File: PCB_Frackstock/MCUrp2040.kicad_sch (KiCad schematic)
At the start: 32 parts, among them J10 SWD, J6 Conn_01x02_Male, J8 Conn_01x02_Male, U1 RP2040, U2 W25Q128JVSIQ, Y3 12MHz

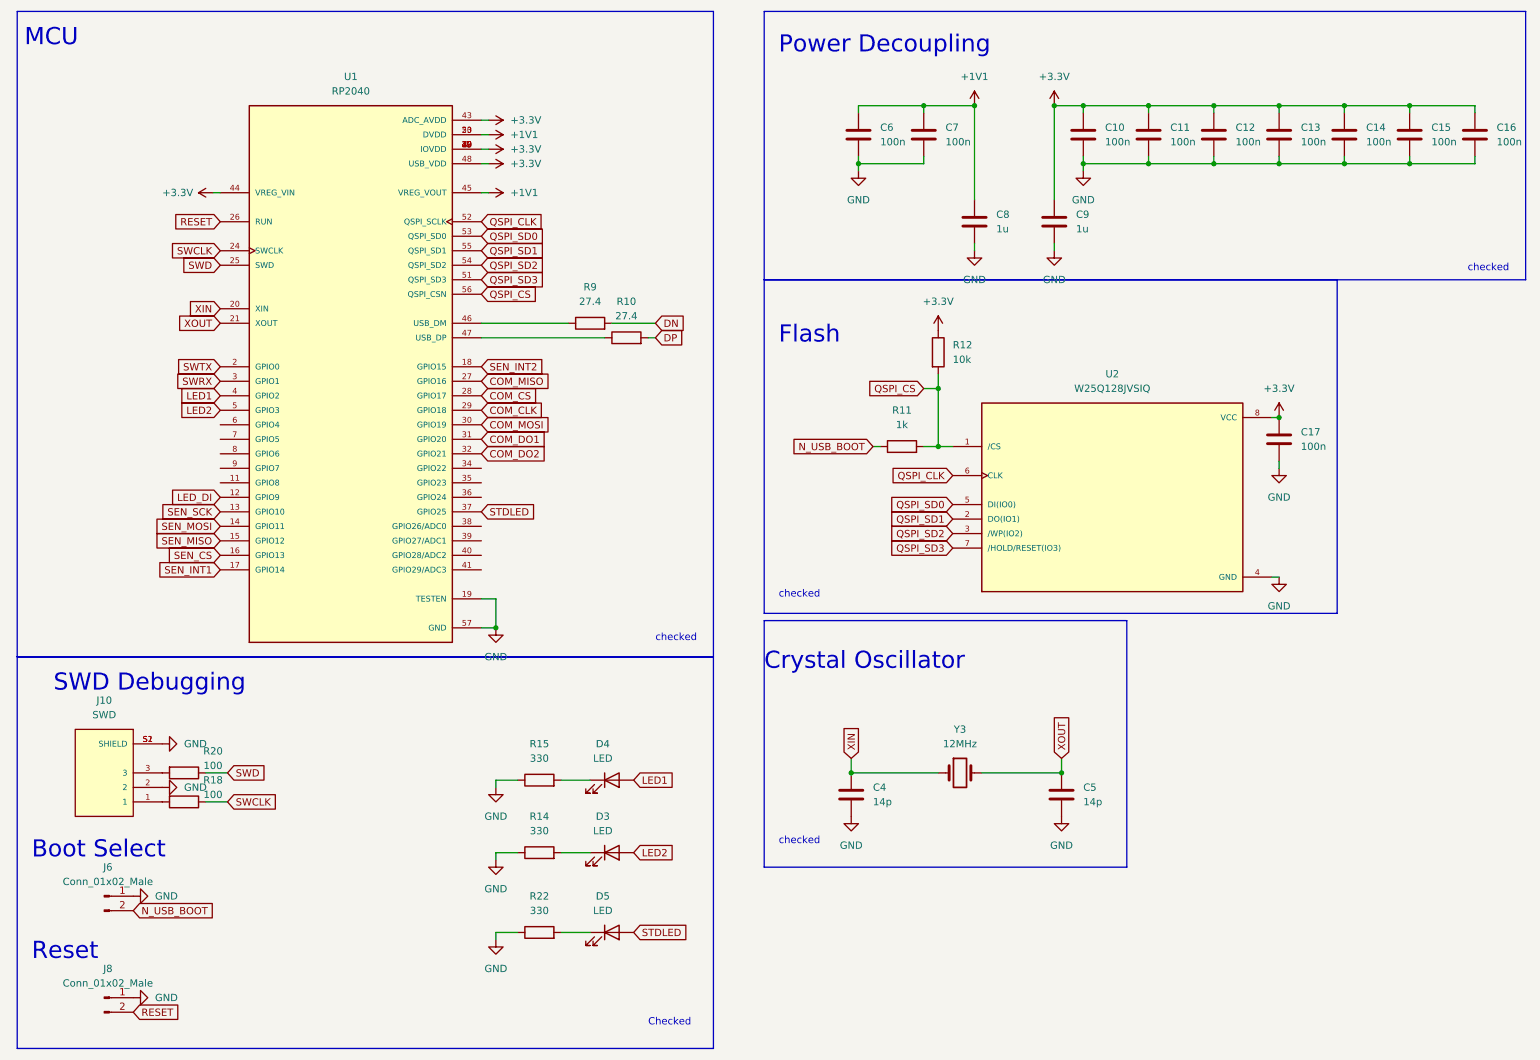
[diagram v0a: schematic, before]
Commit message: Schema_fertig
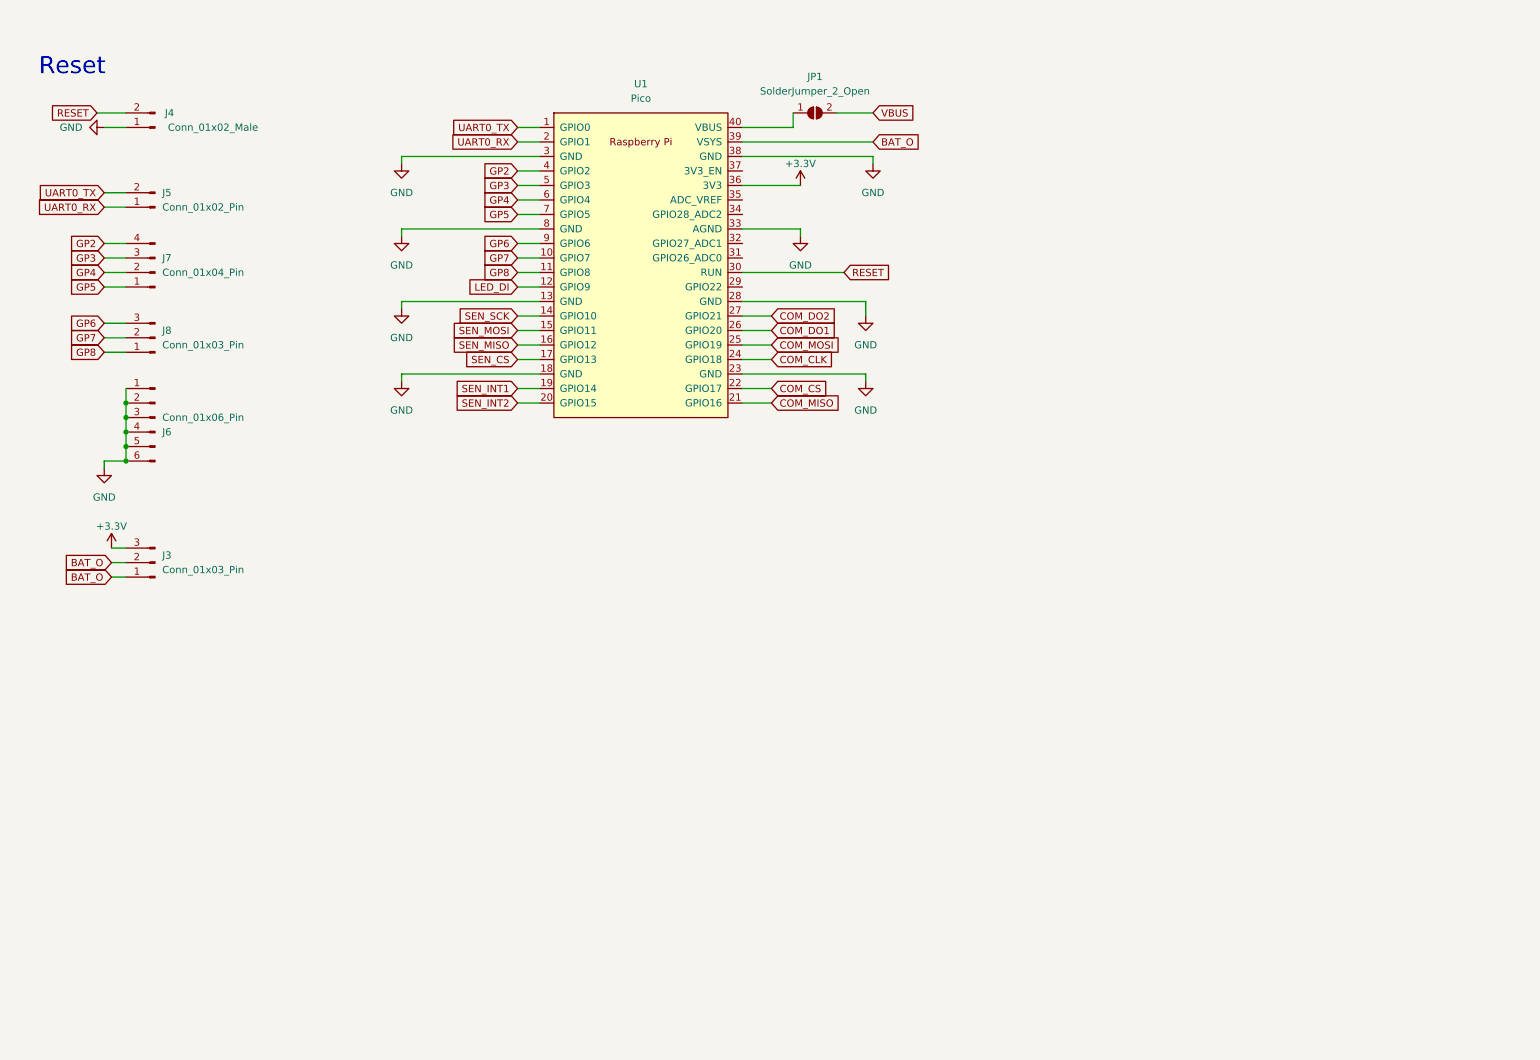
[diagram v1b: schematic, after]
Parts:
- removed C10, C11, C12, C13, C14, C15, C16, C17, C6, C7: 100n, Capacitor_SMD:C_0603_1608Metric_Pad1.08x0.95mm_HandSolder, symbol Device:C
- removed C4, C5: 14p, Capacitor_SMD:C_0603_1608Metric_Pad1.08x0.95mm_HandSolder, symbol Device:C
- removed C8, C9: 1u, Capacitor_SMD:C_0603_1608Metric_Pad1.08x0.95mm_HandSolder, symbol Device:C
- removed D3, D4, D5: LED, LED_SMD:LED_0603_1608Metric_Pad1.05x0.95mm_HandSolder, symbol Device:LED
- removed J10: SWD, SnapEDA Library:JST_SM03B-SRSS-TB(LF)(SN), symbol SM03B-SRSS-TB_LF__SN_:SM03B-SRSS-TB(LF)(SN)
- removed J6, J8: Conn_01x02_Male, Connector_PinHeader_2.54mm:PinHeader_1x02_P2.54mm_Vertical, symbol Connector:Conn_01x02_Male
- removed R10, R9: 27.4, Resistor_SMD:R_0603_1608Metric_Pad0.98x0.95mm_HandSolder, symbol Device:R
- removed R11: 1k, Resistor_SMD:R_0603_1608Metric_Pad0.98x0.95mm_HandSolder, symbol Device:R
- removed R12: 10k, Resistor_SMD:R_0603_1608Metric_Pad0.98x0.95mm_HandSolder, symbol Device:R
- removed R14, R15, R22: 330, Resistor_SMD:R_0603_1608Metric_Pad0.98x0.95mm_HandSolder, symbol Device:R
- removed R18, R20: 100, Resistor_SMD:R_0603_1608Metric_Pad0.98x0.95mm_HandSolder, symbol Device:R
- removed U1: RP2040, SnapEDA Library:QFN40P700X700X90-57N, symbol RP2040:RP2040
- removed U2: W25Q128JVSIQ, SnapEDA Library:SOIC127P790X216-8N, symbol W25Q128JVSIQ:W25Q128JVSIQ
- removed Y3: 12MHz, Crystal:Crystal_SMD_5032-2Pin_5.0x3.2mm, symbol Device:Crystal
- added J3, J8: Conn_01x03_Pin, Connector_PinHeader_2.54mm:PinHeader_1x03_P2.54mm_Vertical, symbol Connector:Conn_01x03_Pin
- added J4: Conn_01x02_Male, Connector_PinHeader_2.54mm:PinHeader_1x02_P2.54mm_Vertical, symbol Connector:Conn_01x02_Male
- added J5: Conn_01x02_Pin, Connector_PinHeader_2.54mm:PinHeader_1x02_P2.54mm_Vertical, symbol Connector:Conn_01x02_Pin
- added J6: Conn_01x06_Pin, Connector_PinHeader_2.54mm:PinHeader_1x06_P2.54mm_Vertical, symbol Connector:Conn_01x06_Pin
- added J7: Conn_01x04_Pin, Connector_PinHeader_2.54mm:PinHeader_1x04_P2.54mm_Vertical, symbol Connector:Conn_01x04_Pin
- added JP1: SolderJumper_2_Open, Jumper:SolderJumper-2_P1.3mm_Open_RoundedPad1.0x1.5mm, symbol Jumper:SolderJumper_2_Open
- added U1: Pico, Frack:RPi_Pico_SMD_ohne_Debug, symbol Frack:Pico_ohne_Debug
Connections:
- net +3.3V: now also J3.3 (Pin_3), U1.36 (3V3)
- net COM_CLK: now also U1.24 (GPIO18)
- net COM_CS: now also U1.22 (GPIO17)
- net COM_DO1: now also U1.26 (GPIO20)
- net COM_DO2: now also U1.27 (GPIO21)
- net COM_MISO: now also U1.21 (GPIO16)
- net COM_MOSI: now also U1.25 (GPIO19)
- net GND: now also J4.1 (Pin_1), J6.1 (Pin_1), J6.2 (Pin_2), J6.3 (Pin_3), J6.4 (Pin_4), J6.5 (Pin_5), J6.6 (Pin_6), U1.13 (GND), U1.18 (GND), U1.23 (GND), U1.28 (GND), U1.3 (GND), U1.33 (AGND), U1.38 (GND), U1.8 (GND)
- net LED_DI: now also U1.12 (GPIO9)
- net RESET: now also J4.2 (Pin_2), U1.30 (RUN)
- net SEN_CS: now also U1.17 (GPIO13)
- net SEN_INT1: now also U1.19 (GPIO14)
- net SEN_INT2: now also U1.20 (GPIO15)
- net SEN_MISO: now also U1.16 (GPIO12)
- net SEN_MOSI: now also U1.15 (GPIO11)
- net SEN_SCK: now also U1.14 (GPIO10)
- new net: JP1.1 (A), U1.40 (VBUS)
- new net BAT_O: J3.1 (Pin_1), J3.2 (Pin_2), U1.39 (VSYS)
- new net GP2: J7.4 (Pin_4), U1.4 (GPIO2)
- new net GP3: J7.3 (Pin_3), U1.5 (GPIO3)
- new net GP4: J7.2 (Pin_2), U1.6 (GPIO4)
- new net GP5: J7.1 (Pin_1), U1.7 (GPIO5)
- new net GP6: J8.3 (Pin_3), U1.9 (GPIO6)
- new net GP7: J8.2 (Pin_2), U1.10 (GPIO7)
- new net GP8: J8.1 (Pin_1), U1.11 (GPIO8)
- new net UART0_RX: J5.1 (Pin_1), U1.2 (GPIO1)
- new net UART0_TX: J5.2 (Pin_2), U1.1 (GPIO0)
- new net VBUS: JP1.2 (B)
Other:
- note removed: "Boot Select"
- note removed: "Checked"
- note removed: "Crystal Oscillator"
- note removed: "Flash"
- note removed: "MCU"
- note removed: "Power Decoupling"
- note removed: "SWD Debugging"
- note removed: "checked"

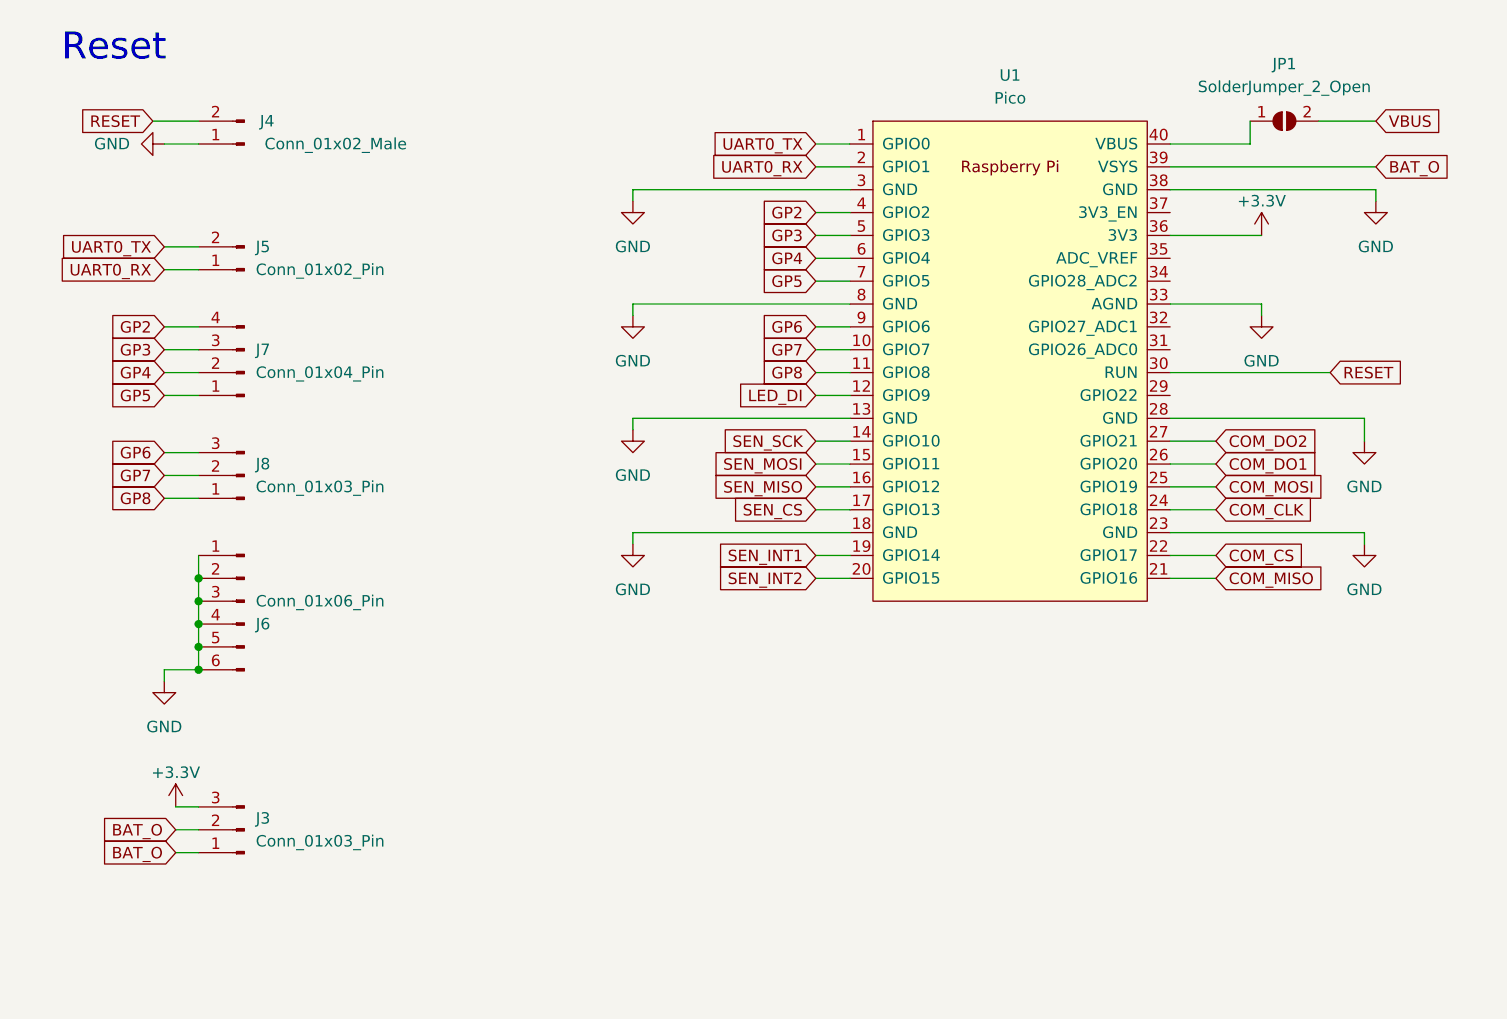
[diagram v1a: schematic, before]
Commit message: Layout Fertig
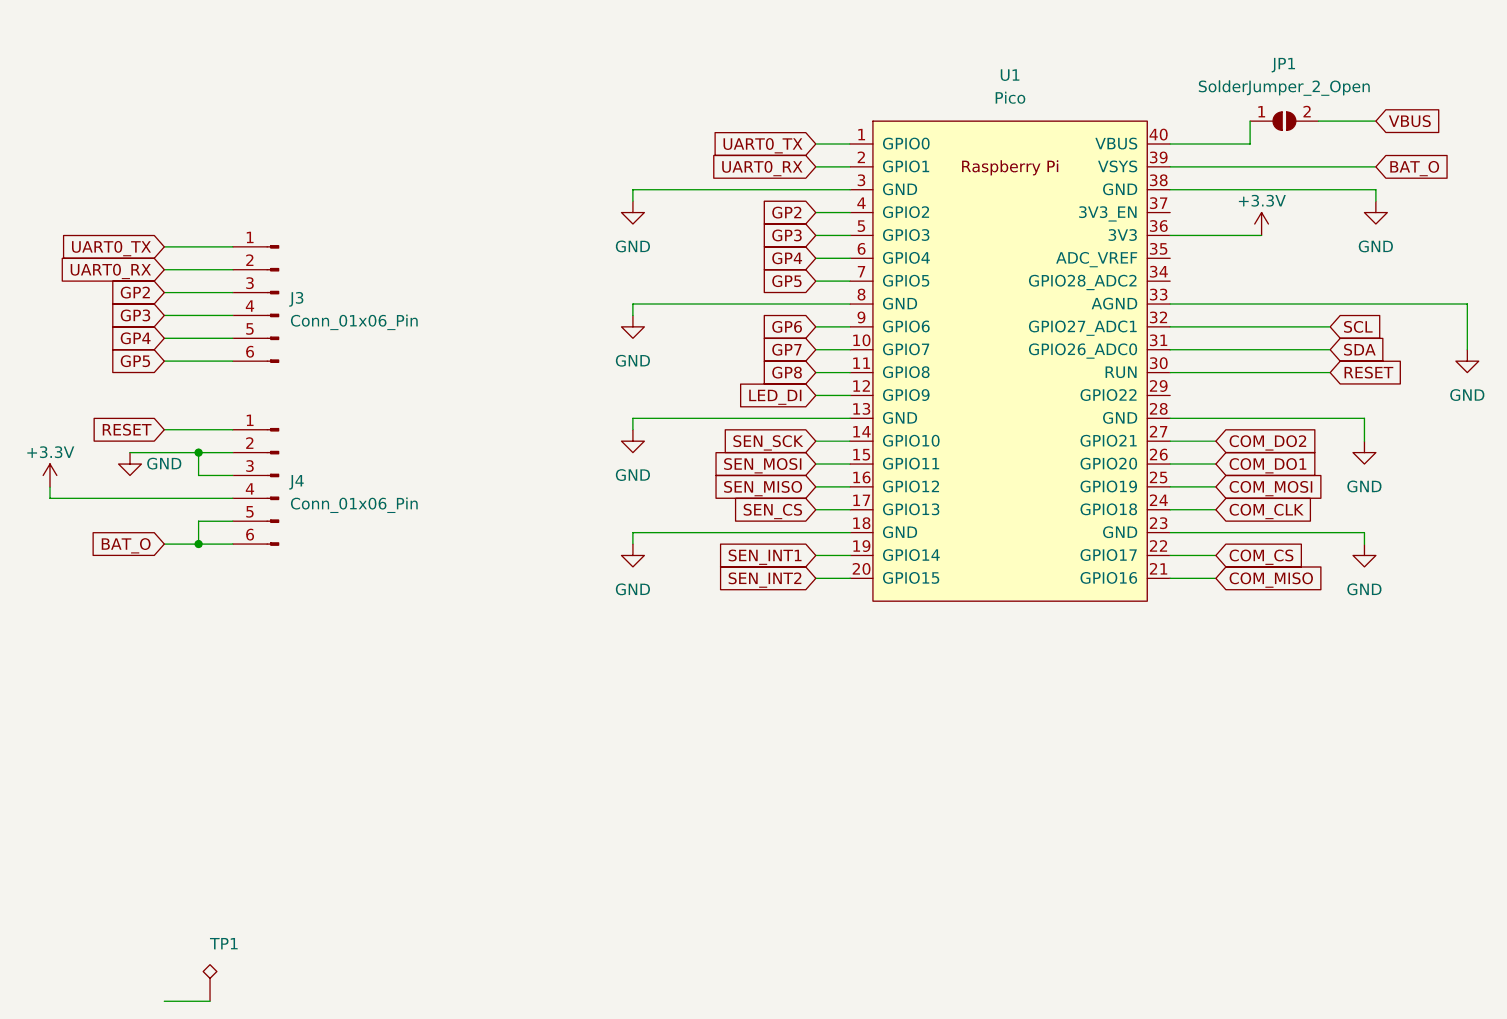
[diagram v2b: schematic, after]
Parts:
- removed J3, J8: Conn_01x03_Pin, Connector_PinHeader_2.54mm:PinHeader_1x03_P2.54mm_Vertical, symbol Connector:Conn_01x03_Pin
- removed J4: Conn_01x02_Male, Connector_PinHeader_2.54mm:PinHeader_1x02_P2.54mm_Vertical, symbol Connector:Conn_01x02_Male
- removed J5: Conn_01x02_Pin, Connector_PinHeader_2.54mm:PinHeader_1x02_P2.54mm_Vertical, symbol Connector:Conn_01x02_Pin
- removed J6: Conn_01x06_Pin, Connector_PinHeader_2.54mm:PinHeader_1x06_P2.54mm_Vertical, symbol Connector:Conn_01x06_Pin
- removed J7: Conn_01x04_Pin, Connector_PinHeader_2.54mm:PinHeader_1x04_P2.54mm_Vertical, symbol Connector:Conn_01x04_Pin
- added J3, J4: Conn_01x06_Pin, Frack:PinHeader_2x03_P2.54mm_Vertical_SMD_kleiner, symbol Connector:Conn_01x06_Pin
- added TP1: TestPoint_Alt, TestPoint:TestPoint_Pad_D1.5mm, symbol Connector:TestPoint_Alt
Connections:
- net +3.3V: now also J4.4 (Pin_4)
- net BAT_O: now also J4.5 (Pin_5), J4.6 (Pin_6)
- net GND: now also J4.2 (Pin_2), J4.3 (Pin_3)
- net GP2: now also J3.3 (Pin_3)
- net GP3: now also J3.4 (Pin_4)
- net GP4: now also J3.5 (Pin_5)
- net GP5: now also J3.6 (Pin_6)
- net RESET: now also J4.1 (Pin_1)
- net UART0_RX: now also J3.2 (Pin_2)
- net UART0_TX: now also J3.1 (Pin_1)
- net SDA: now reaches U1.31 (GPIO26_ADC0)
- net SCL: now reaches U1.32 (GPIO27_ADC1)
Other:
- note removed: "Reset"
